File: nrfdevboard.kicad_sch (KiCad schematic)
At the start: 17 parts, among them J2 Conn_01x07_Pin, P1 USB_C_Plug_USB2.0, U1 MDBT50Q-P1MV2, U3 AP2112K-3.3TRG1, Y1 O_32.768kHz

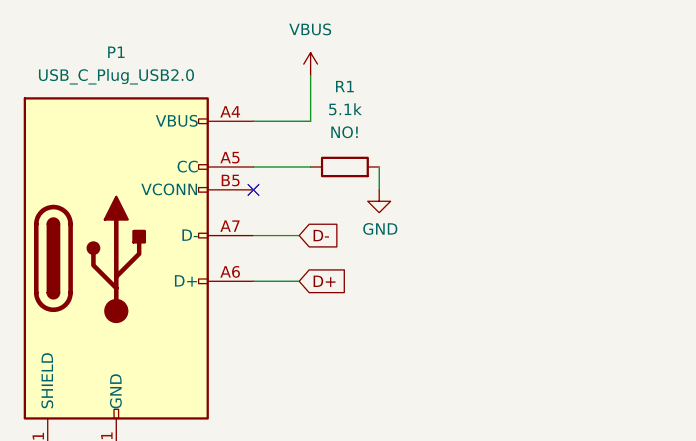
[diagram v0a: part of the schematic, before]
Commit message: Minor tweaks
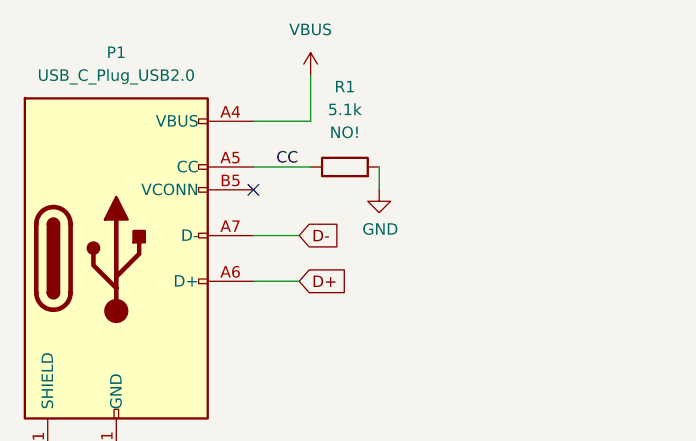
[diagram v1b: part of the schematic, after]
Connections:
- net CC: now reaches P1.A5 (CC), R1.1
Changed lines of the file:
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@@
+		)
+	)
+	(label "CC"
+		(at 54.61 43.18 0)
+		(effects
+			(font
+				(size 1.27 1.27)
+			)
+			(justify left bottom)
 		)
 	)
